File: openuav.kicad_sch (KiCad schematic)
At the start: 64 parts, among them J1 Conn_01x01, J10 Conn_01x01, J11 Conn_01x01, J12 Conn_01x01, J13 Conn_01x01, J14 Conn_01x01, J15 Conn_01x01, J16 Conn_01x01, J17 Conn_01x01, J18 Conn_01x01, J19 Conn_01x01, J2 Conn_01x01, J20 Conn_01x01, J21 Conn_01x01, J22 Conn_01x01, J23 Conn_01x01, J24 Conn_01x01, J25 Conn_01x01, J26 Conn_01x01, J27 Conn_01x01, J28 Conn_01x01, J29 Conn_01x01, J3 Conn_01x01, J30 Conn_01x01, J31 Conn_01x01, J32 Conn_01x01, J4 Conn_01x01, J5 Conn_01x01, J6 Conn_01x01, J7 Conn_01x01, J8 Conn_01x01, J9 Conn_01x01, J99 USB_C_Receptacle_USB2.0, U1 STM32G431CBUx, U2 AT7456E, U3 LSM6DSR, U4 LPS22HH, U5 L78L33_SOT89, U6 W25N01GVZEIG, U7 L78L05_SOT89, U8 L78L09_SOT89

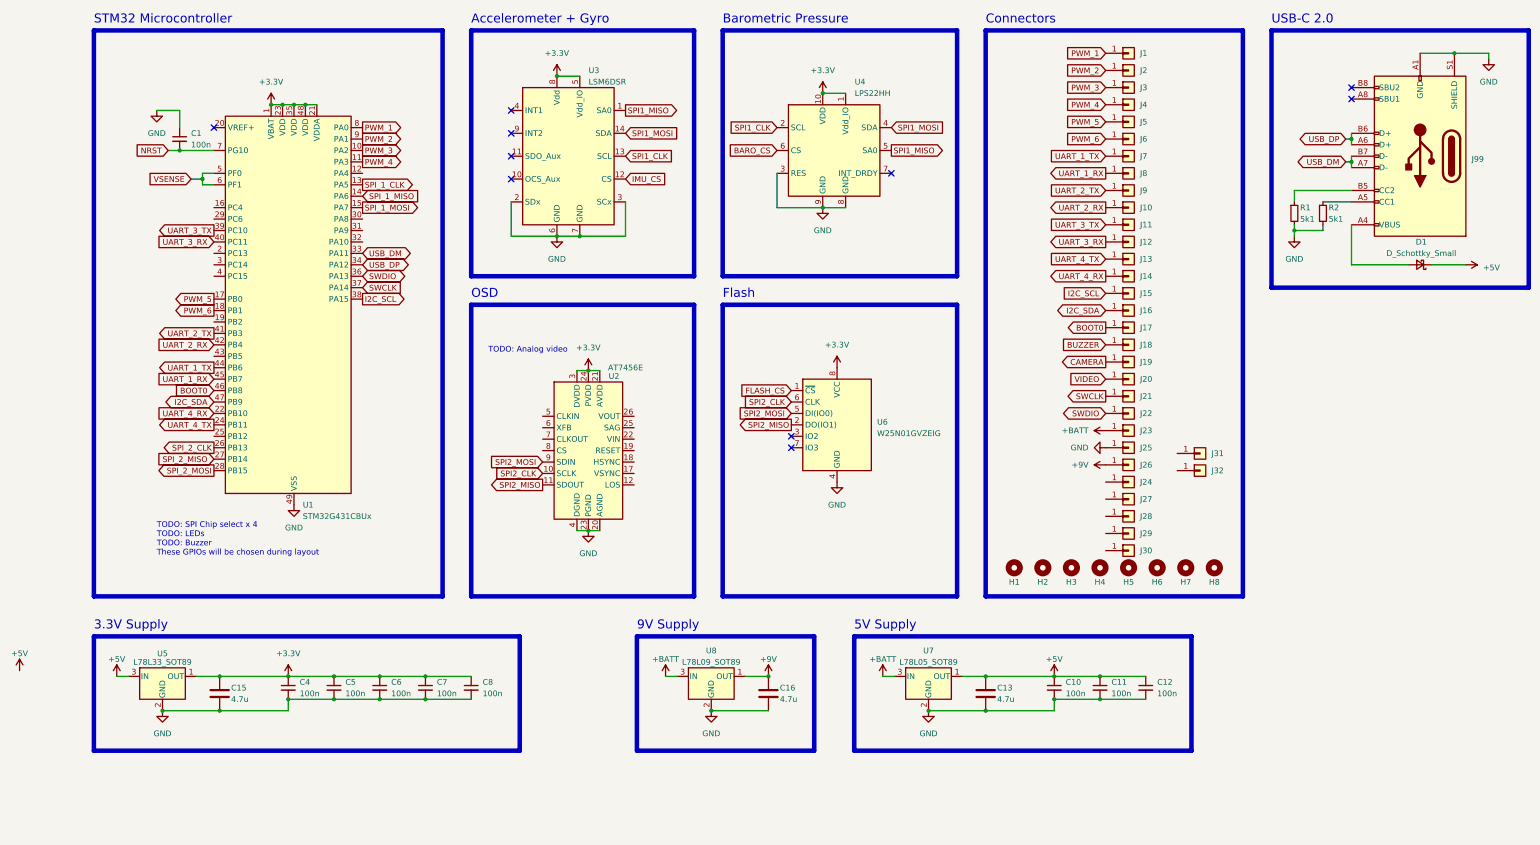
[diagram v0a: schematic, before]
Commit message: start to rethink power supplies
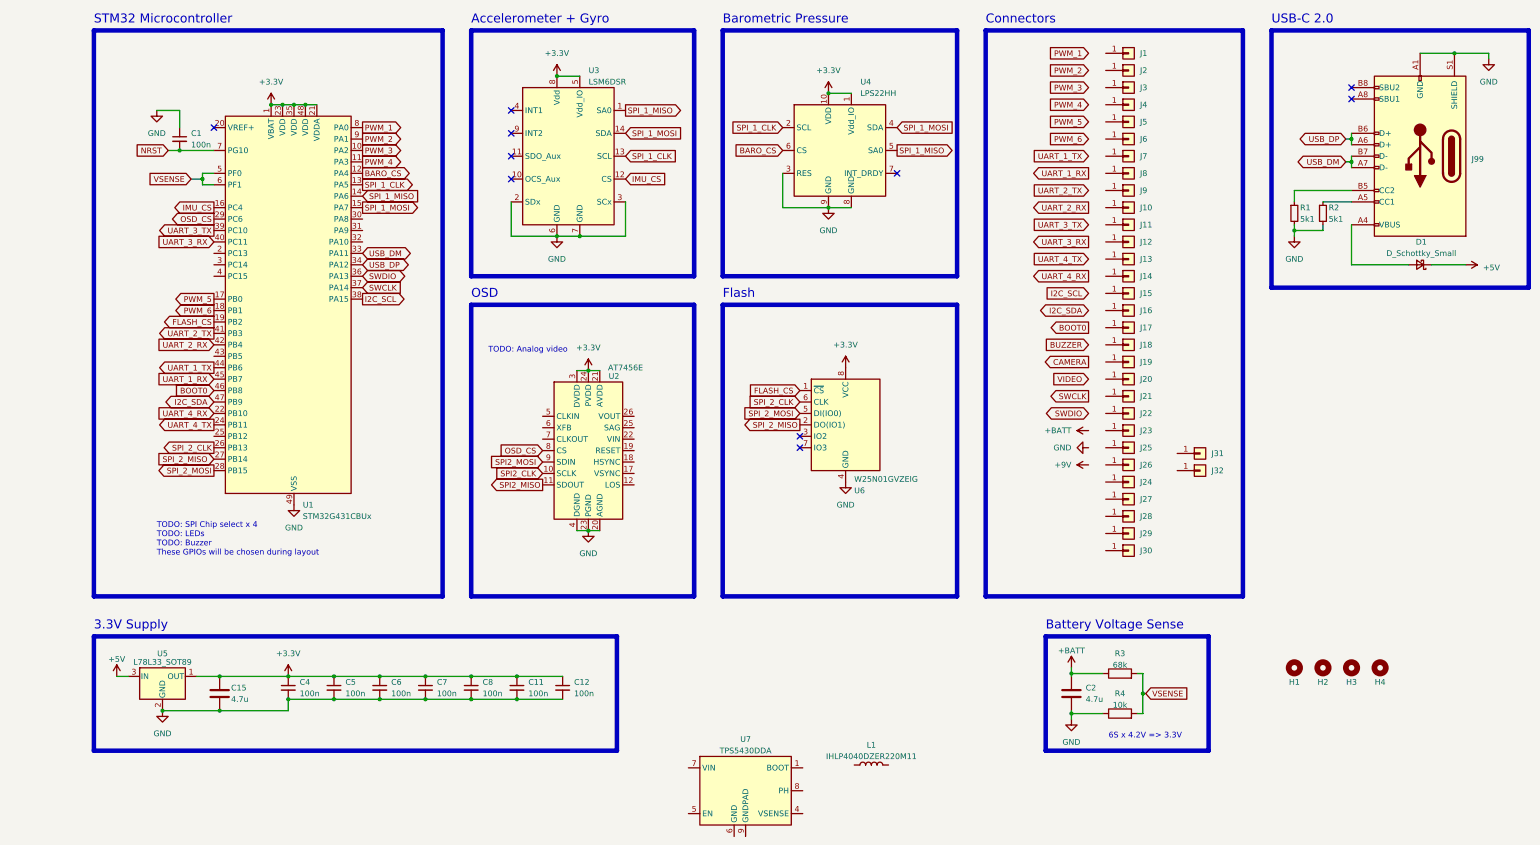
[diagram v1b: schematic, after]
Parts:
- removed C10: 100n, Capacitor_SMD:C_0402_1005Metric, symbol Device:C_Small
- removed C13, C16: 4.7u, Capacitor_SMD:C_0603_1608Metric, symbol Device:C
- removed H5, H6, H7, H8: MountingHole, MountingHole:MountingHole_3.2mm_M3, symbol Mechanical:MountingHole
- removed U7: L78L05_SOT89, Package_TO_SOT_SMD:SOT-89-3, symbol Regulator_Linear:L78L05_SOT89
- removed U8: L78L09_SOT89, Package_TO_SOT_SMD:SOT-89-3, symbol Regulator_Linear:L78L09_SOT89
- added C2: 4.7u, Capacitor_SMD:C_0603_1608Metric, symbol Device:C
- added L1: IHLP4040DZER220M11, Inductor_SMD:L_Vishay_IHLP-4040, symbol Device:L
- added R3: 68k, Resistor_SMD:R_0402_1005Metric, symbol Device:R
- added R4: 10k, Resistor_SMD:R_0402_1005Metric, symbol Device:R
- added U7: TPS5430DDA, Package_SO:TI_SO-PowerPAD-8_ThermalVias, symbol Regulator_Switching:TPS5430DDA
- J1, J10, J11, J12, J13, J14, J15, J16, J17, J18, J19, J2, J20, J21, J22, J23, J24, J25, J26, J27, J28, J29, J3, J30, J31, J32, J4, J5, J6, J7, J8, J9: footprint TestPoint:TestPoint_Pad_2.0x2.0mm -> Connector_Custom_Pads:TestPoint_Pad_2.0x3.0mm
- R1, R2: footprint (none) -> Resistor_SMD:R_0402_1005Metric
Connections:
- net SPI1_CLK is gone; now on net SPI_1_CLK: U3.13 (SCL), U4.2 (SCL)
- net SPI1_MISO is gone; now on net SPI_1_MISO: U3.1 (SA0), U4.5 (SA0)
- net SPI1_MOSI is gone; now on net SPI_1_MOSI: U3.14 (SDA), U4.4 (SDA)
- net +3V3: now also C11.1, C12.1
- net +5V: no longer C11.1, C12.1
- net +9V: no longer J26.1 (Pin_1)
- net +BATT: now also C2.1, R3.1; no longer J23.1 (Pin_1)
- net BARO_CS: now also U1.12 (PA4)
- net BOOT0: no longer J17.1 (Pin_1)
- net BUZZER: no longer J18.1 (Pin_1)
- net CAMERA: no longer J19.1 (Pin_1)
- net FLASH_CS: now also U1.19 (PB2)
- net GND: now also C2.2, R4.1; no longer J25.1 (Pin_1)
- net I2C_SCL: no longer J15.1 (Pin_1)
- net I2C_SDA: no longer J16.1 (Pin_1)
- net IMU_CS: now also U1.16 (PC4)
- net PWM_1: no longer J1.1 (Pin_1)
- net PWM_2: no longer J2.1 (Pin_1)
- net PWM_3: no longer J3.1 (Pin_1)
- net PWM_4: no longer J4.1 (Pin_1)
- net PWM_5: no longer J5.1 (Pin_1)
- net PWM_6: no longer J6.1 (Pin_1)
- net SPI2_CLK: no longer U6.6 (CLK)
- net SPI2_MISO: no longer U6.2 (DO(IO1))
- net SPI2_MOSI: no longer U6.5 (DI(IO0))
- net SPI_2_CLK: now also U6.6 (CLK)
- net SPI_2_MISO: now also U6.2 (DO(IO1))
- net SPI_2_MOSI: now also U6.5 (DI(IO0))
- net SWCLK: no longer J21.1 (Pin_1)
- net SWDIO: no longer J22.1 (Pin_1)
- net UART_1_RX: no longer J8.1 (Pin_1)
- net UART_1_TX: no longer J7.1 (Pin_1)
- net UART_2_RX: no longer J10.1 (Pin_1)
- net UART_2_TX: no longer J9.1 (Pin_1)
- net UART_3_RX: no longer J12.1 (Pin_1)
- net UART_3_TX: no longer J11.1 (Pin_1)
- net UART_4_RX: no longer J14.1 (Pin_1)
- net UART_4_TX: no longer J13.1 (Pin_1)
- net VIDEO: no longer J20.1 (Pin_1)
- net VSENSE: now also R3.2, R4.2
- net OSD_CS: now reaches U2.8 (CS)
- net OSD_CS: now also U1.29 (PC6)
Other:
- note added: "6S x 4.2V => 3.3V"
- note added: "Battery Voltage Sense"
- note removed: "5V Supply"
- note removed: "9V Supply"
- moved on the sheet: C11, C12, H1, H2, H3, H4, U4, U6
